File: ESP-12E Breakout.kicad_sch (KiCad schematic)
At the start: 6 parts, among them J3 Conn_01x08_Pin, J4 Conn_01x08_Pin, J5 Conn_01x06_Pin, U1 ESP-12E

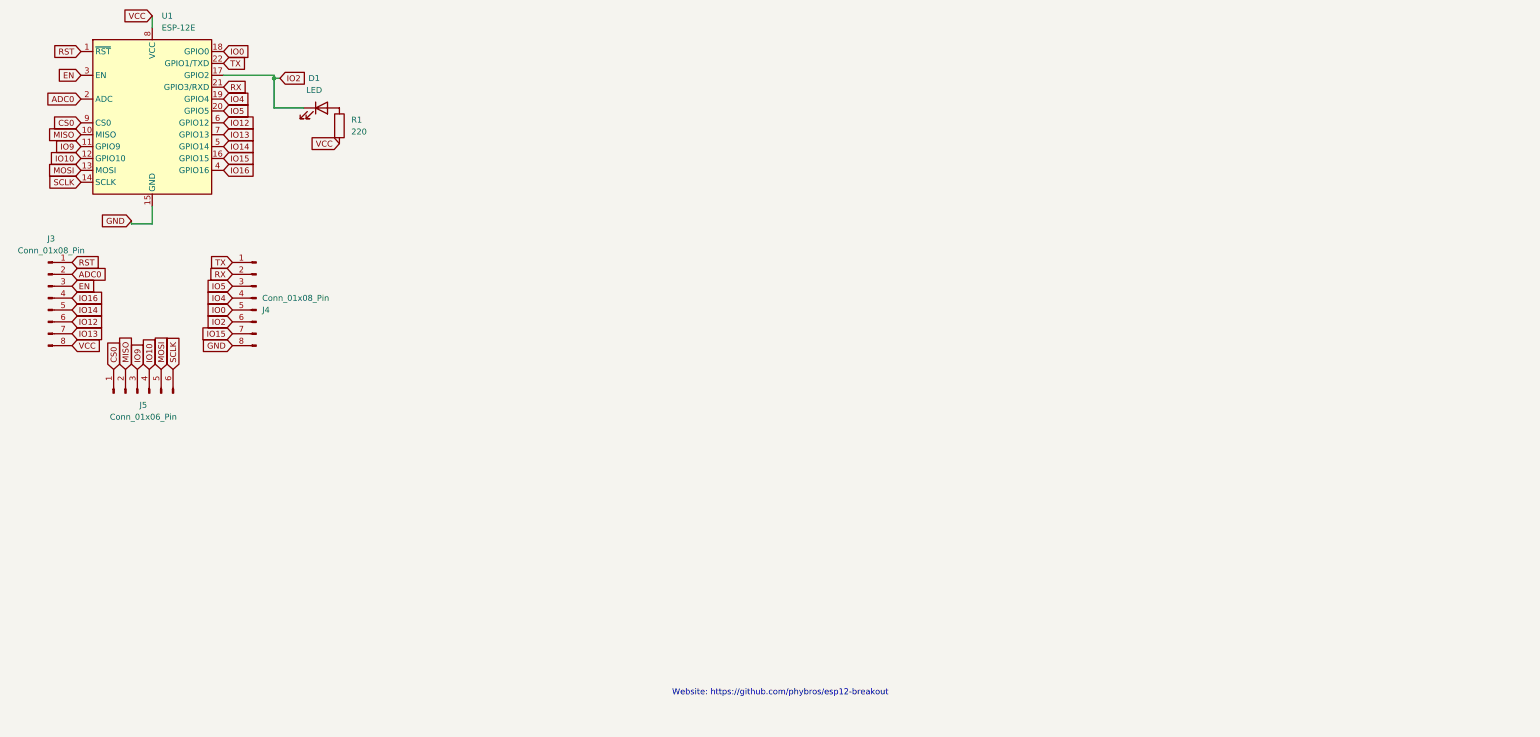
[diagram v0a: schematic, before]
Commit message: Add files via upload
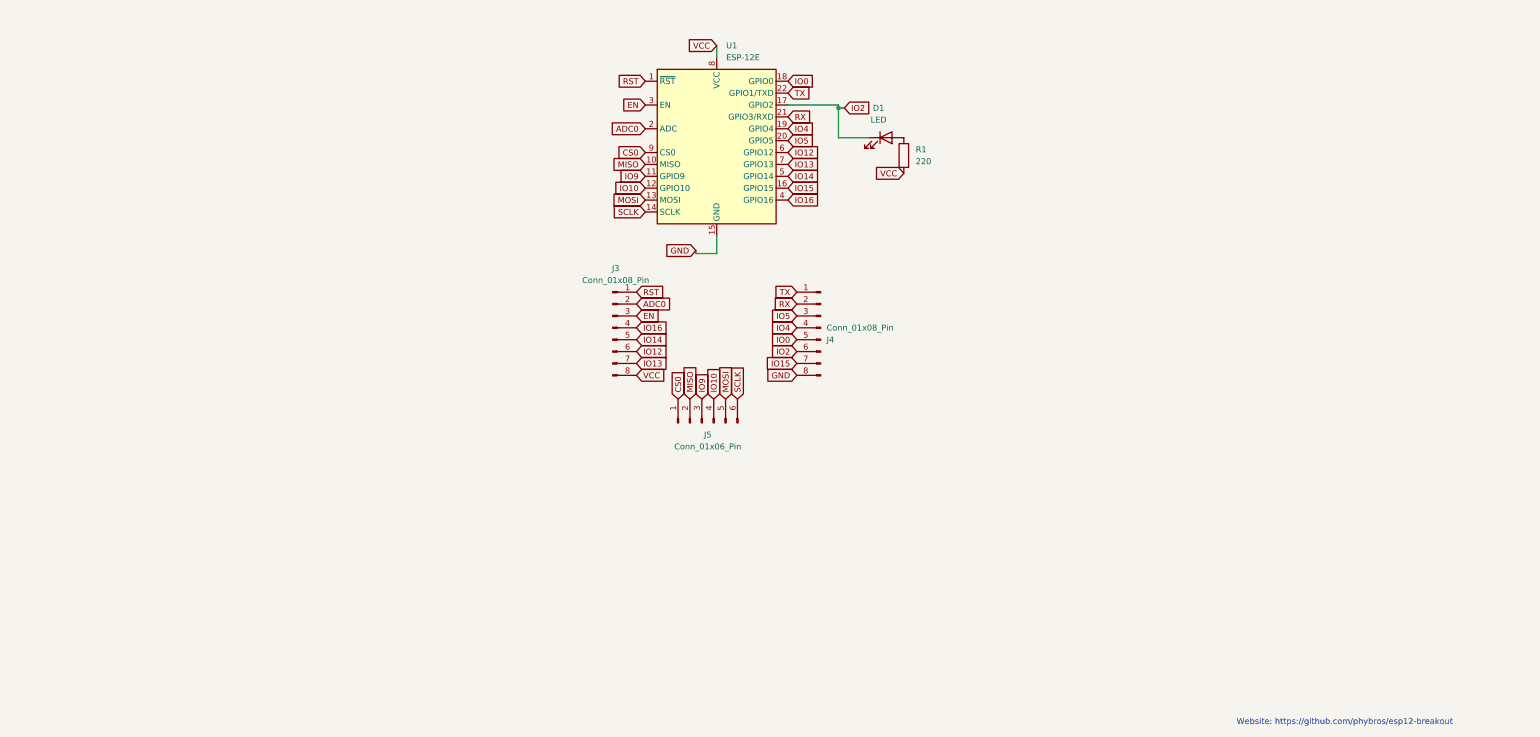
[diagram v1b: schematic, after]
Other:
- moved on the sheet: D1, J3, J4, J5, R1, U1
